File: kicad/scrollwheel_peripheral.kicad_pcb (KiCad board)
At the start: 2 copper layers, 71.5 x 38 mm, 9 parts, among them J1 Conn_01x14_Socket, J2 Conn_01x14_Socket, J3 Conn_01x05_Socket

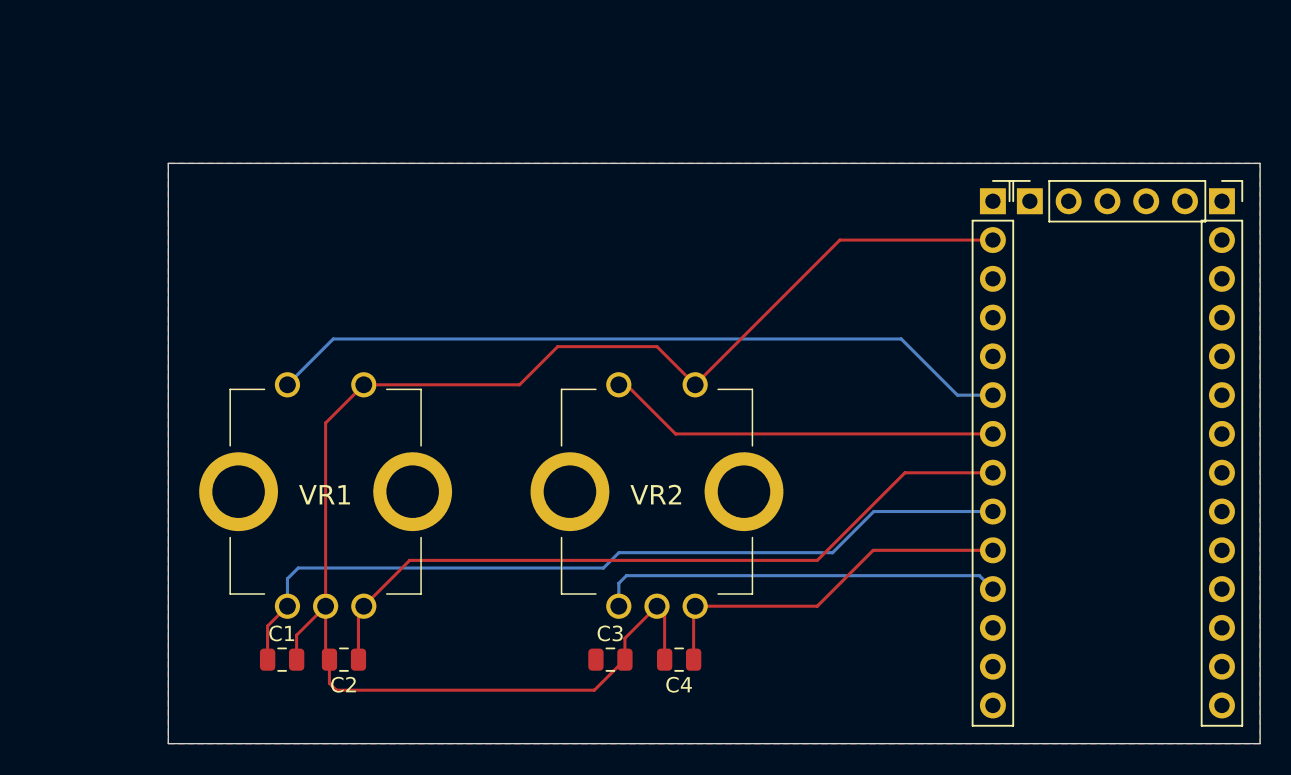
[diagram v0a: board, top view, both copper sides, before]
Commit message: Misc changes
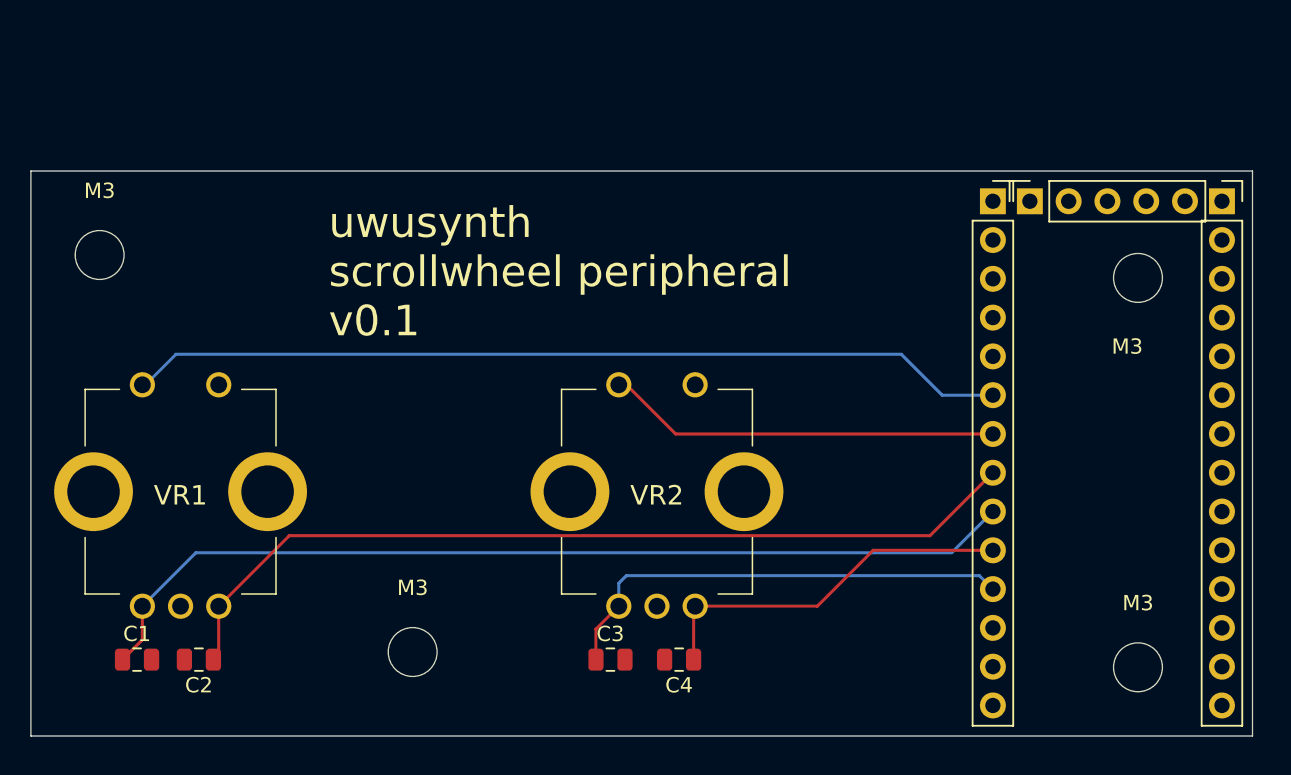
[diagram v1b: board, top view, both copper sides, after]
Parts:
- added M3: MountingHole_3.2mm_M3, MountingHole:MountingHole_3.2mm_M3, F.Cu at (114.5, 60.5)
- added M3: MountingHole_3.2mm_M3, MountingHole:MountingHole_3.2mm_M3, F.Cu at (46.5, 59.0)
- added M3: MountingHole_3.2mm_M3, MountingHole:MountingHole_3.2mm_M3, F.Cu at (114.5, 86.0)
- added M3: MountingHole_3.2mm_M3, MountingHole:MountingHole_3.2mm_M3, F.Cu at (67.0, 85.0)
- moved C1 9.50 mm to (49.0, 85.5)
- moved C2 9.50 mm to (53.0, 85.5)
- moved VR1 9.50 mm to (49.3, 67.5)
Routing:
- net GND: track 100.6 -> 0.71 mm
- net Net-(J1-Pin_8): track 48.5 -> 58.0 mm
- net Net-(J1-Pin_6): track 49.0 -> 57.6 mm
- net Net-(J1-Pin_9): track 53.9 -> 62.3 mm
- net Net-(J1-Pin_11): track 26.6 -> 30.7 mm
- removed copper zone on B.Cu, net GND
- removed copper zone on F.Cu, net GND
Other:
- board size 71.5 x 38 mm -> 80 x 37 mm
- board text added: "uwusynth scrollwheel peripheral v0.1"

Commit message: Misc
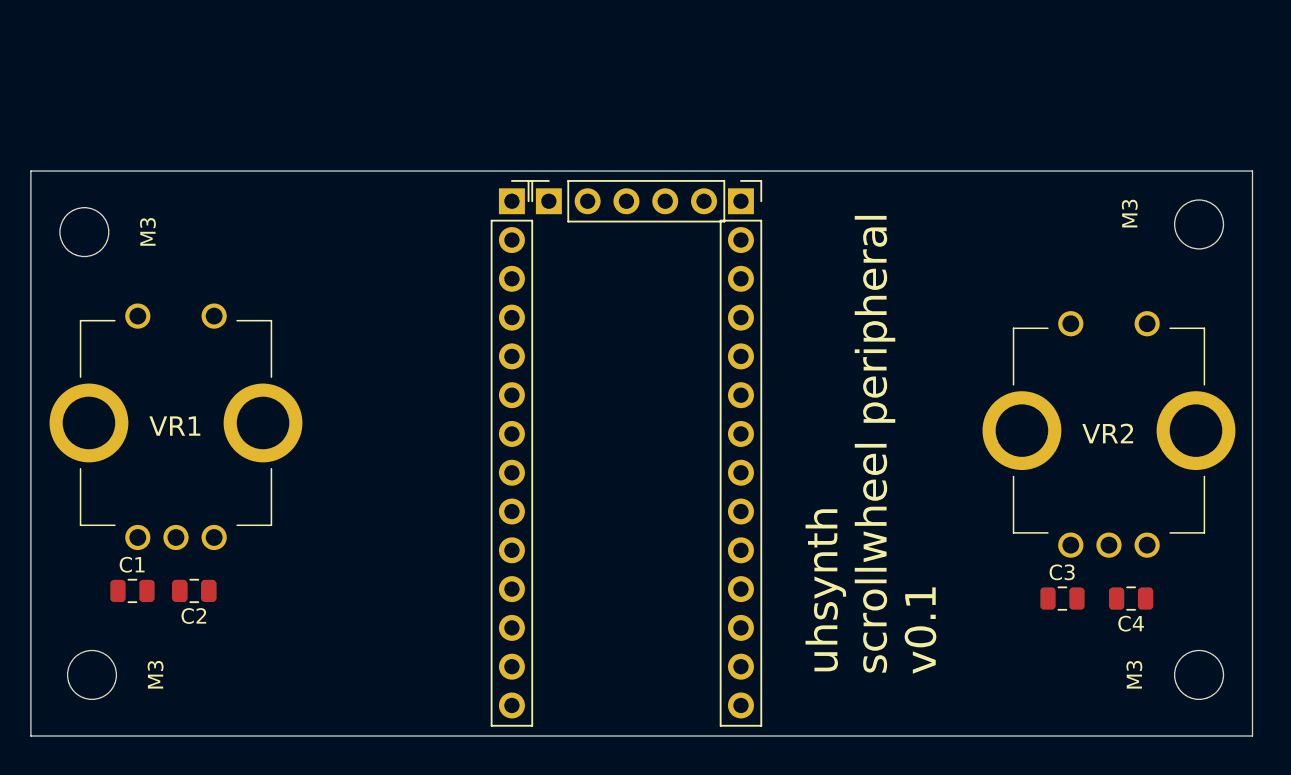
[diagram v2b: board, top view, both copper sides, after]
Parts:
- moved J1 31.5 mm to (73.5, 55.5)
- moved J2 31.5 mm to (88.5, 55.5)
- moved J3 31.5 mm to (75.9, 55.5)
- moved C3 29.9 mm to (109.5, 81.5)
- moved C4 29.9 mm to (114.0, 81.5)
- moved VR2 29.9 mm to (110.1, 63.5)
- moved M3 21.1 mm to (46.0, 86.5), turned to -90 degrees
- moved M3 5.32 mm to (118.5, 57.0), turned to -90 degrees
- moved C1 4.51 mm to (48.6, 81.0)
- moved C2 4.51 mm to (52.7, 81.0)
- moved VR1 4.51 mm to (49.0, 63.0)
- moved M3 4.03 mm to (118.5, 86.5), turned to 90 degrees
- moved M3 1.80 mm to (45.5, 57.5), turned to -90 degrees
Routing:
- net Net-(J1-Pin_9): track 62.3 -> 0.00 mm
- net Net-(J1-Pin_8): track 58.0 -> 0.00 mm
- net Net-(J1-Pin_6): track 57.6 -> 0.00 mm
- net Net-(J1-Pin_11): track 30.7 -> 0.00 mm
- net Net-(J1-Pin_7): track 25.8 -> 0.00 mm
- net Net-(J1-Pin_10): track 24.6 -> 0.00 mm
- net GND: track 0.71 -> 0.00 mm
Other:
- board text added: "uhsynth scrollwheel peripheral v0.1"
- board text removed: "uwusynth scrollwheel peripheral v0.1"
